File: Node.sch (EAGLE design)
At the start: 69 parts, among them J1 AVR_SPI_PRG_6NS, J2 M04X2, Q1 PMR280UN, Q2 PMR280UN, Q3 PMR280UN, U1 ATMEGA32U4, U2 BLUETOOTH-RN41", U4 L3GD20, U9 RCLAMP0502A, X1 USBSMD

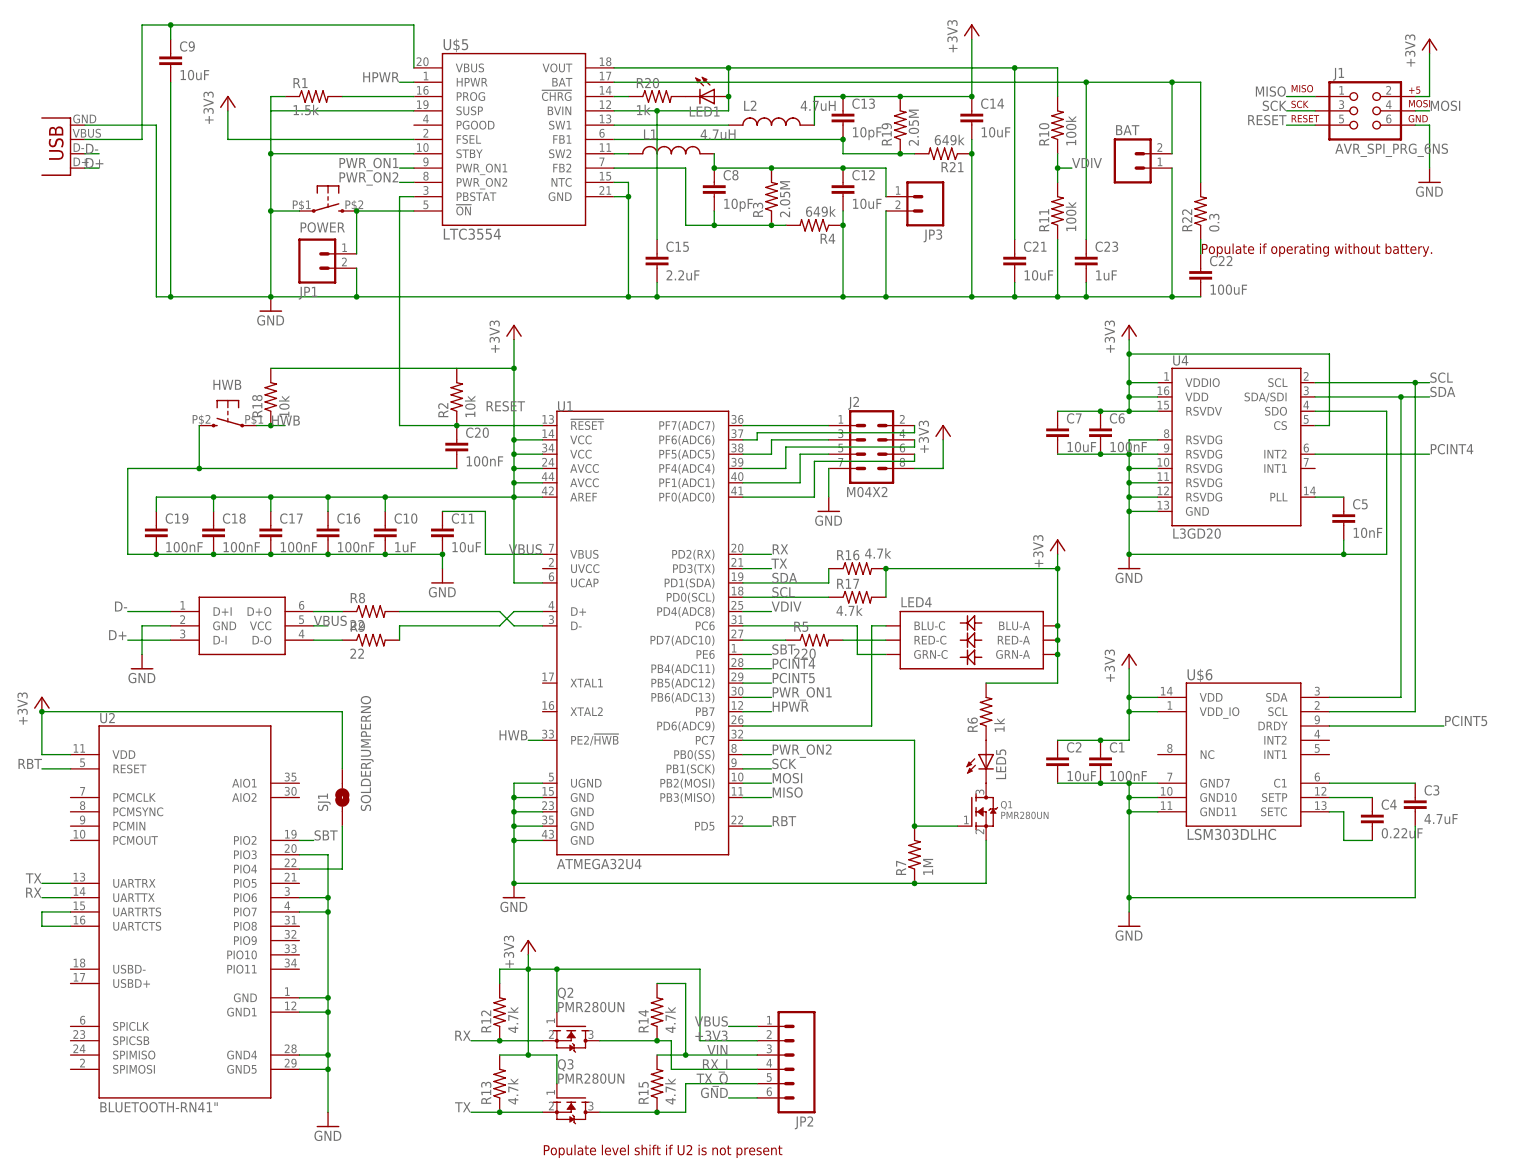
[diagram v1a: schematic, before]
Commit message: pass ERC
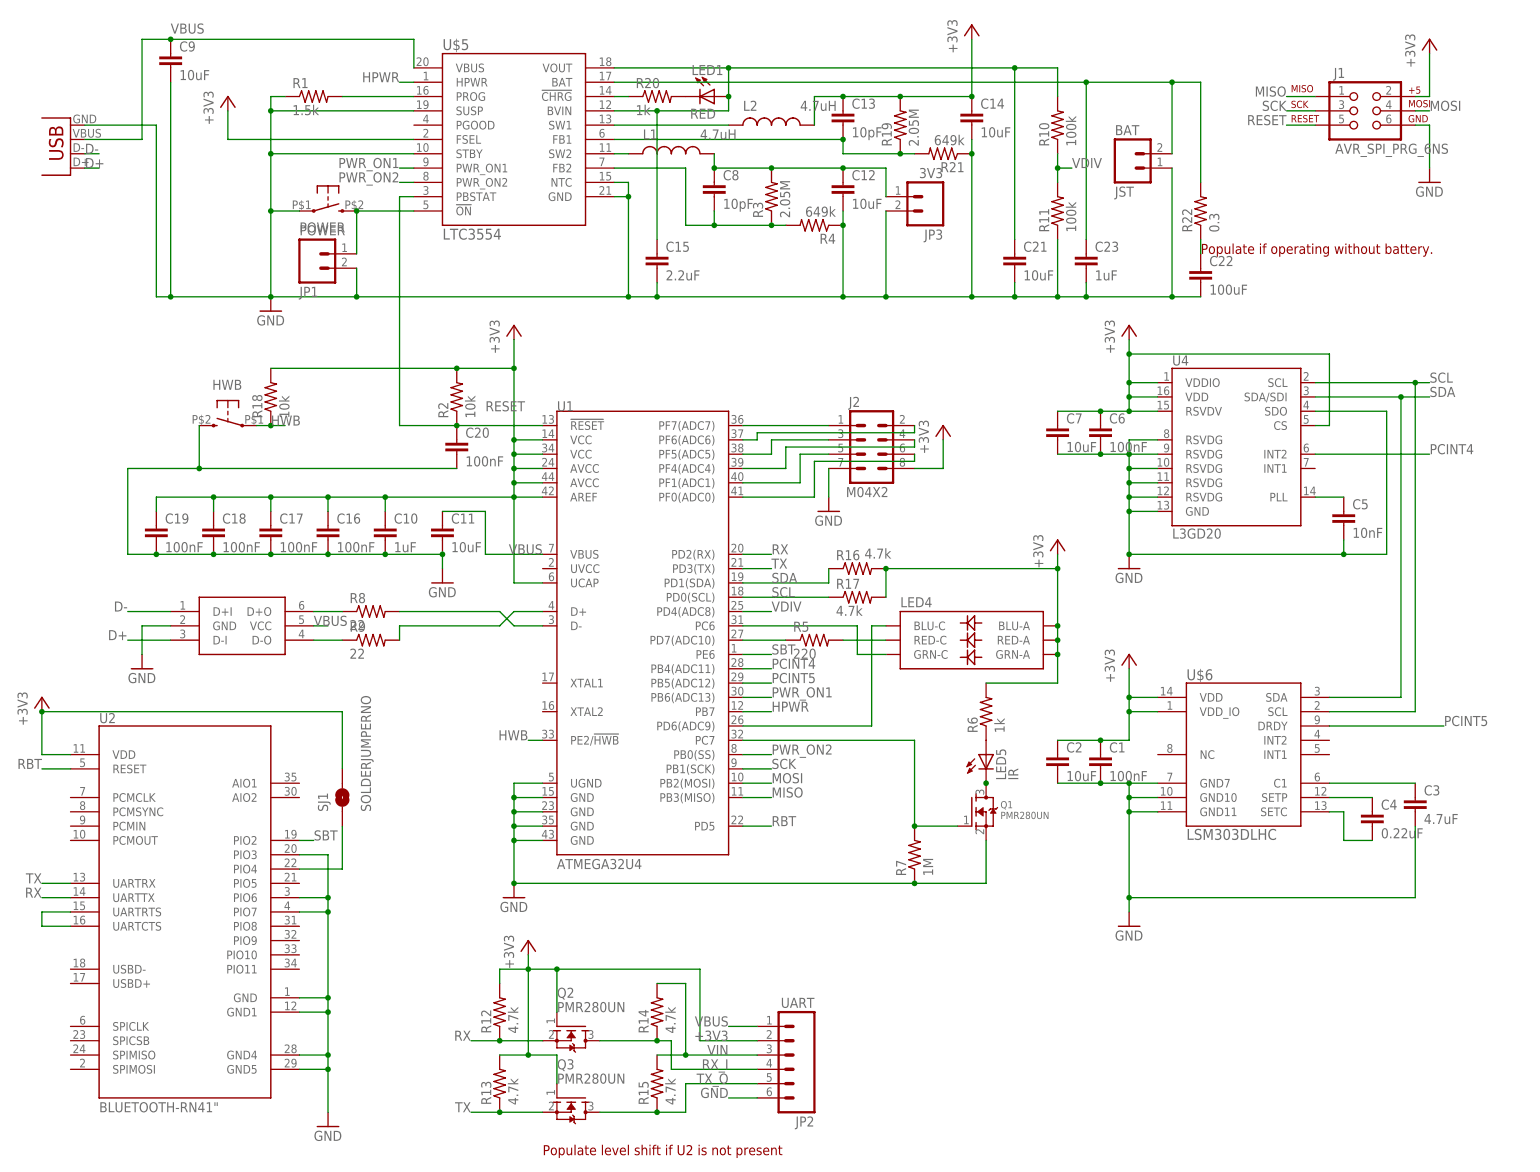
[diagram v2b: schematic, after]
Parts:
- BAT: value (none) -> JST
- JP1: value (none) -> POWER
- JP2: value (none) -> UART
- JP3: value (none) -> 3V3
- LED1: value (none) -> RED
- LED5: value (none) -> IR
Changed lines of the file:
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@@
 </classes>
 <parts>
-<part name="FRAME1" library="frames" deviceset="FRAME_A_L" device=""/>
+<part name="FRAME1" library="frames" deviceset="FRAME_A_L" device="" value="Tracker"/>
 <part name="U1" library="adjacent-reality" deviceset="ATMEGA32U4" device=""/>
 <part name="U4" library="adjacent-reality" deviceset="L3GD20" device=""/>
@@
 <part name="GND4" library="supply1" deviceset="GND" device=""/>
 <part name="X1" library="SparkFun" deviceset="USB" device="SMD"/>
-<part name="BAT" library="SparkFun" deviceset="M02" device="-JST-2MM-SMT"/>
+<part name="BAT" library="SparkFun" deviceset="M02" device="-JST-2MM-SMT" value="JST"/>
 <part name="C9" library="SparkFun" deviceset="CAP" device="0603-CAP" value="10uF"/>
 <part name="GND5" library="supply1" deviceset="GND" device=""/>
@@
 <part name="+3V5" library="supply1" deviceset="+3V3" device=""/>
 <part name="+3V6" library="supply1" deviceset="+3V3" device=""/>
-<part name="LED5" library="SparkFun" deviceset="LED" device="0603"/>
+<part name="LED5" library="SparkFun" deviceset="LED" device="0603" value="IR"/>
 <part name="R6" library="SparkFun" deviceset="RESISTOR" device="0402-RES" value="1k"/>
 <part name="R7" library="SparkFun" deviceset="RESISTOR" device="0402-RES" value="1M"/>
@@
 <part name="U9" library="adjacent-reality" deviceset="RCLAMP0502A" device=""/>
 <part name="GND9" library="supply1" deviceset="GND" device=""/>
-<part name="LED1" library="SparkFun" deviceset="LED" device="0603"/>
+<part name="LED1" library="SparkFun" deviceset="LED" device="0603" value="RED"/>
 <part name="R20" library="SparkFun" deviceset="RESISTOR" device="0402-RES" value="1k"/>
 <part name="R10" library="SparkFun" deviceset="RESISTOR" device="0402-RES" value="100k"/>
@@
 <part name="J2" library="SparkFun" deviceset="M04X2" device=""/>
 <part name="+3V9" library="supply1" deviceset="+3V3" device=""/>
-<part name="JP2" library="SparkFun" deviceset="M06" device="SIP"/>
+<part name="JP2" library="SparkFun" deviceset="M06" device="SIP" value="UART"/>
 <part name="U$5" library="adjacent-reality" deviceset="LTC3554" device=""/>
 <part name="R1" library="SparkFun" deviceset="RESISTOR" device="0402-RES" value="1.5k"/>
@@
 <part name="R21" library="SparkFun" deviceset="RESISTOR" device="0402-RES" value="649k"/>
 <part name="C14" library="SparkFun" deviceset="CAP" device="0603-CAP" value="10uF"/>
-<part name="JP3" library="SparkFun-Connectors" deviceset="M02" device="PTH"/>
+<part name="JP3" library="SparkFun-Connectors" deviceset="M02" device="PTH" value="3V3"/>
 <part name="C15" library="SparkFun" deviceset="CAP" device="0402-CAP" value="2.2uF"/>
 <part name="C21" library="SparkFun" deviceset="CAP" device="0402-CAP" value="10uF"/>
@@
 <part name="L1" library="adjacent-reality" deviceset="INDUCTOR" device="VLS2016" value="4.7uH"/>
 <part name="L2" library="adjacent-reality" deviceset="INDUCTOR" device="VLS2016" value="4.7uH"/>
-<part name="JP1" library="SparkFun-Connectors" deviceset="M02" device="PTH"/>
+<part name="JP1" library="SparkFun-Connectors" deviceset="M02" device="PTH" value="POWER"/>
 </parts>
 <sheets>
@@
 <instance part="U9" gate="G$1" x="50.8" y="99.06"/>
 <instance part="GND9" gate="1" x="154.94" y="119.38"/>
-<instance part="LED1" gate="G$1" x="134.62" y="193.04" rot="R270"/>
+<instance part="LED1" gate="G$1" x="134.62" y="193.04" smashed="yes" rot="R270">
+<attribute name="NAME" x="130.556" y="196.85" size="1.778" layer="95"/>
+<attribute name="VALUE" x="130.302" y="189.103" size="1.778" layer="96"/>
+</instance>
 <instance part="R20" gate="G$1" x="124.46" y="193.04"/>
 <instance part="R10" gate="G$1" x="195.58" y="187.96" rot="R90"/>
@@
 <wire x1="58.42" y1="193.04" x2="55.88" y2="193.04" width="0.1524" layer="91"/>
 <wire x1="55.88" y1="193.04" x2="55.88" y2="190.5" width="0.1524" layer="91"/>
-<pinref part="U$5" gate="G$1" pin="SUSP"/>
 <wire x1="55.88" y1="190.5" x2="55.88" y2="182.88" width="0.1524" layer="91"/>
 <wire x1="55.88" y1="182.88" x2="55.88" y2="172.72" width="0.1524" layer="91"/>
 <wire x1="55.88" y1="172.72" x2="55.88" y2="157.48" width="0.1524" layer="91"/>
-<wire x1="81.28" y1="190.5" x2="55.88" y2="190.5" width="0.1524" layer="91"/>
 <pinref part="U$5" gate="G$1" pin="STBY"/>
 <wire x1="81.28" y1="182.88" x2="55.88" y2="182.88" width="0.1524" layer="91"/>
@@
 <wire x1="71.12" y1="162.56" x2="71.12" y2="157.48" width="0.1524" layer="91"/>
 <junction x="71.12" y="157.48"/>
+<pinref part="U$5" gate="G$1" pin="SUSP"/>
+<wire x1="81.28" y1="190.5" x2="55.88" y2="190.5" width="0.1524" layer="91"/>
+<junction x="55.88" y="190.5"/>
 </segment>
 <segment>
@@
 <junction x="76.2" y="121.92"/>
 <pinref part="R2" gate="G$1" pin="2"/>
-<wire x1="88.9" y1="144.78" x2="99.06" y2="144.78" width="0.1524" layer="91"/>
 <junction x="99.06" y="144.78"/>
 <wire x1="88.9" y1="144.78" x2="55.88" y2="144.78" width="0.1524" layer="91"/>
 <pinref part="R18" gate="G$1" pin="2"/>
+<wire x1="99.06" y1="144.78" x2="88.9" y2="144.78" width="0.1524" layer="91"/>
+<junction x="88.9" y="144.78"/>
 </segment>
 <segment>
@@
 </segment>
 <segment>
-<pinref part="C9" gate="G$1" pin="1"/>
-<wire x1="38.1" y1="205.74" x2="38.1" y2="203.2" width="0.1524" layer="91"/>
-<wire x1="38.1" y1="205.74" x2="33.02" y2="205.74" width="0.1524" layer="91"/>
-<wire x1="33.02" y1="205.74" x2="33.02" y2="185.42" width="0.1524" layer="91"/>
-<pinref part="X1" gate="G$1" pin="VBUS"/>
-<wire x1="33.02" y1="185.42" x2="22.86" y2="185.42" width="0.1524" layer="91"/>
-<pinref part="U$5" gate="G$1" pin="VBUS"/>
-<wire x1="38.1" y1="205.74" x2="81.28" y2="205.74" width="0.1524" layer="91"/>
-<wire x1="81.28" y1="205.74" x2="81.28" y2="198.12" width="0.1524" layer="91"/>
-<junction x="38.1" y="205.74"/>
-</segment>
-<segment>
 <wire x1="63.5" y1="99.06" x2="66.04" y2="99.06" width="0.1524" layer="91"/>
 <label x="63.5" y="99.06" size="1.778" layer="95"/>
@@
 <wire x1="142.24" y1="27.94" x2="137.16" y2="27.94" width="0.1524" layer="91"/>
 <label x="137.16" y="27.94" size="1.778" layer="95" rot="MR0"/>
+</segment>
+<segment>
+<pinref part="X1" gate="G$1" pin="VBUS"/>
+<wire x1="22.86" y1="185.42" x2="33.02" y2="185.42" width="0.1524" layer="91"/>
+<wire x1="33.02" y1="185.42" x2="33.02" y2="203.2" width="0.1524" layer="91"/>
+<pinref part="C9" gate="G$1" pin="1"/>
+<wire x1="33.02" y1="203.2" x2="38.1" y2="203.2" width="0.1524" layer="91"/>
+<pinref part="U$5" gate="G$1" pin="VBUS"/>
+<wire x1="38.1" y1="203.2" x2="81.28" y2="203.2" width="0.1524" layer="91"/>
+<wire x1="81.28" y1="203.2" x2="81.28" y2="198.12" width="0.1524" layer="91"/>
+<junction x="38.1" y="203.2"/>
+<label x="38.1" y="204.216" size="1.778" layer="95"/>
 </segment>
 </net>
@@
 <net name="N$20" class="0">
 <segment>
-<pinref part="LED5" gate="G$1" pin="C"/>
 <pinref part="Q1" gate="G$1" pin="D"/>
 <pinref part="Q1" gate="G$1" pin="D"/>
-</segment>
-</net>
-<net name="N$21" class="0">
-<segment>
-<pinref part="LED5" gate="G$1" pin="A"/>
-<pinref part="R6" gate="G$1" pin="1"/>
+<pinref part="LED5" gate="G$1" pin="C"/>
+<junction x="182.88" y="71.12"/>
 </segment>
 </net>
@@
 </segment>
 </net>
+<net name="N$4" class="0">
+<segment>
+<pinref part="R6" gate="G$1" pin="1"/>
+<pinref part="LED5" gate="G$1" pin="A"/>
+</segment>
+</net>
